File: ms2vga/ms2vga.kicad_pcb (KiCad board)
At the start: 2 copper layers, 34.3 x 31.8 mm, 2 parts, among them J1 DB9_Male_MountingHoles, J2 DB15_Female_HighDensity_Mount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

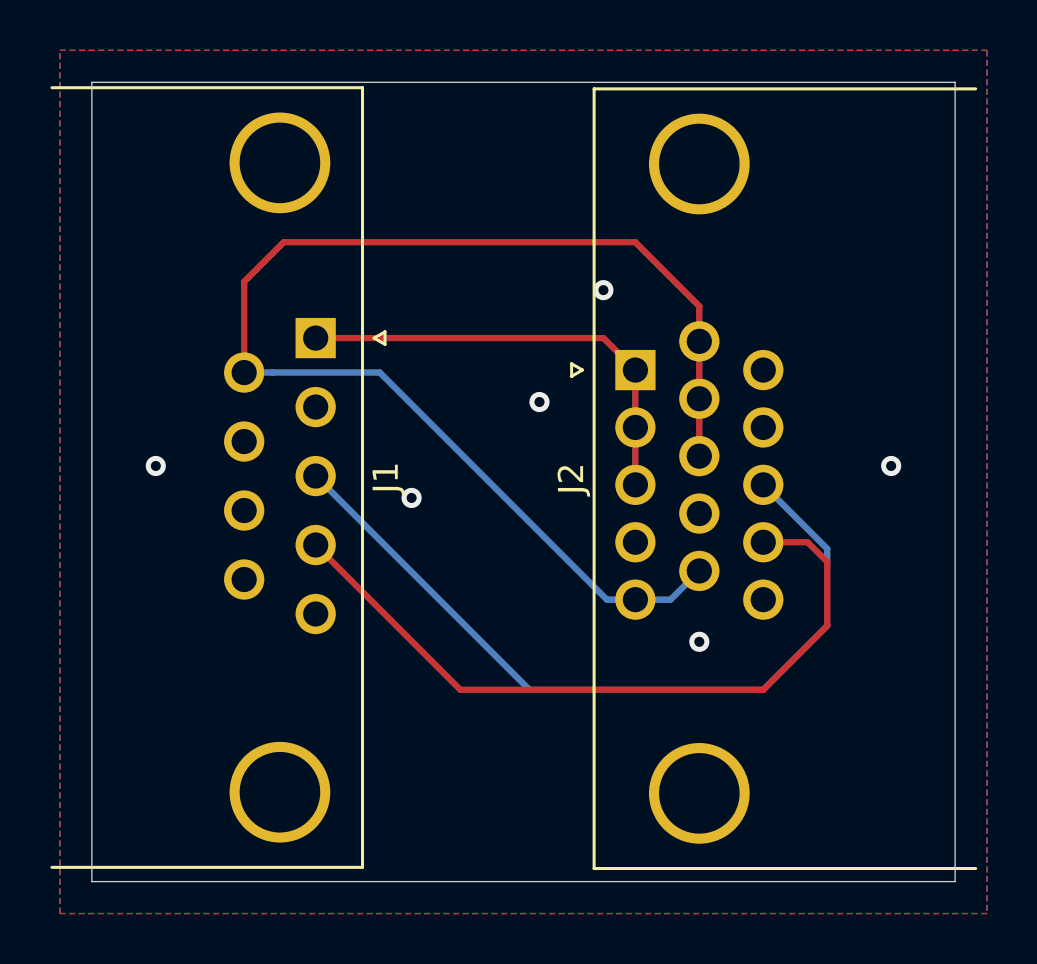
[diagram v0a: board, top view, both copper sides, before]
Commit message: Minor cleanup.
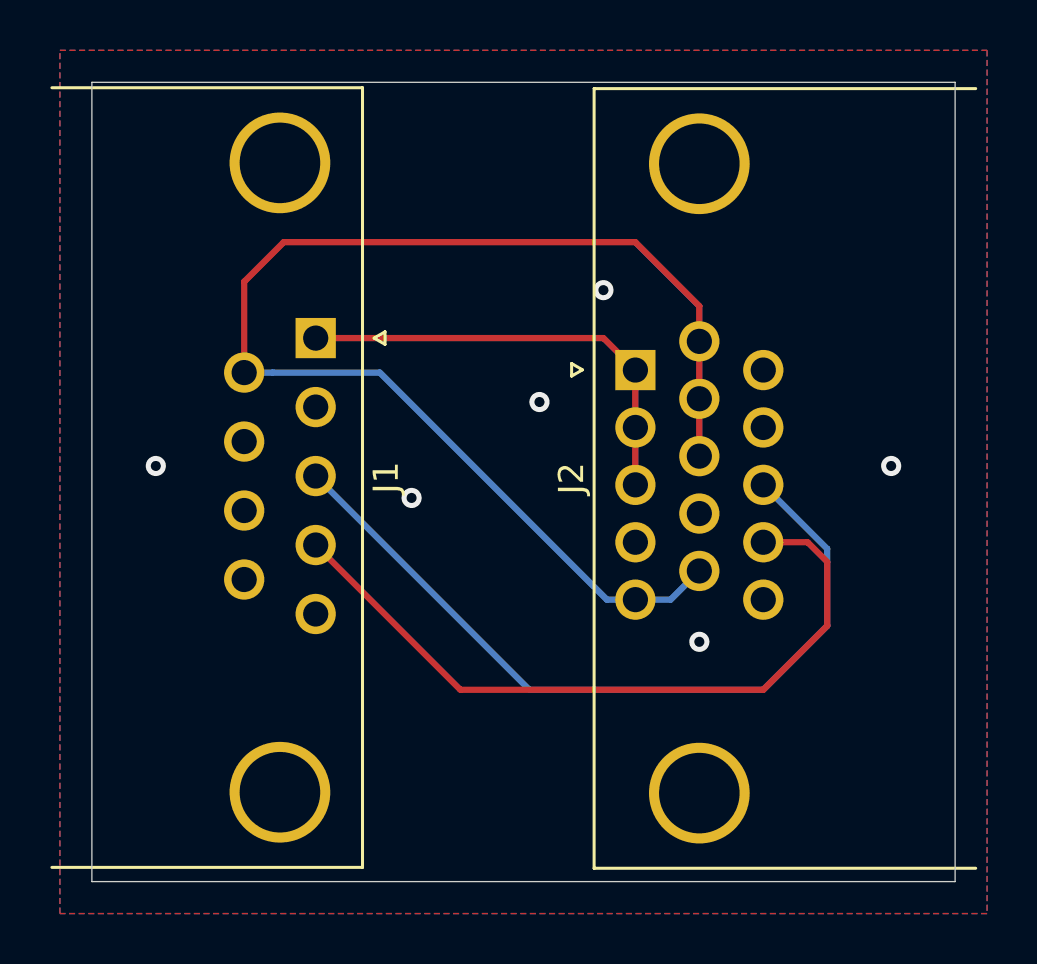
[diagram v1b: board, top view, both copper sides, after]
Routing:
- net Net-(J2-Pad9): vias 0 -> 1
- net /GND: vias 0 -> 1
- net /Chassis: vias 6 -> 4
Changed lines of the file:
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@@
   (general
     (thickness 1.6)
-    (drawings 4)
+    (drawings 6)
     (tracks 34)
     (zones 0)
@@
     (descr "15-pin D-Sub connector, horizontal/angled (90 deg), THT-mount, female, pitch 2.29x1.98mm, pin-PCB-offset 8.35mm, distance of mounting holes 25mm, distance of mounting holes to PCB edge 10.889999999999999mm, see https://disti-assets.s3.amazonaws.com/tonar/files/datasheets/16730.pdf")
     (tags "15-pin D-Sub connector horizontal angled 90deg THT female pitch 2.29x1.98mm pin-PCB-offset 8.35mm mounting-holes-distance 25mm mounting-hole-offset 25mm")
-    (fp_text reference J2 (at -4.315 -2.54 90) (layer F.SilkS)
-      (effects (font (size 1 1) (thickness 0.15)))
-    )
-    (fp_text value DB15_Female_HighDensity_MountingHoles (at -4.315 21.48 90) (layer F.Fab)
-      (effects (font (size 1 1) (thickness 0.15)))
-    )
-    (fp_text user %R (at -4.315 16.98 90) (layer F.Fab)
-      (effects (font (size 1 1) (thickness 0.15)))
-    )
-    (fp_line (start 11.65 -2.1) (end -20.25 -2.1) (layer F.CrtYd) (width 0.05))
-    (fp_line (start 11.65 20.52) (end 11.65 -2.1) (layer F.CrtYd) (width 0.05))
-    (fp_line (start -20.25 20.52) (end 11.65 20.52) (layer F.CrtYd) (width 0.05))
-    (fp_line (start -20.25 -2.1) (end -20.25 20.52) (layer F.CrtYd) (width 0.05))
-    (fp_line (start 0 -2.101325) (end -0.25 -2.534338) (layer F.SilkS) (width 0.12))
-    (fp_line (start 0.25 -2.534338) (end 0 -2.101325) (layer F.SilkS) (width 0.12))
-    (fp_line (start -0.25 -2.534338) (end 0.25 -2.534338) (layer F.SilkS) (width 0.12))
-    (fp_line (start 11.17 -1.64) (end 11.17 13.52) (layer F.SilkS) (width 0.12))
-    (fp_line (start -19.8 -1.64) (end 11.17 -1.64) (layer F.SilkS) (width 0.12))
-    (fp_line (start -19.8 13.52) (end -19.8 -1.64) (layer F.SilkS) (width 0.12))
-    (fp_line (start 9.785 13.58) (end 9.785 2.69) (layer F.Fab) (width 0.1))
-    (fp_line (start 6.585 13.58) (end 6.585 2.69) (layer F.Fab) (width 0.1))
-    (fp_line (start -15.215 13.58) (end -15.215 2.69) (layer F.Fab) (width 0.1))
-    (fp_line (start -18.415 13.58) (end -18.415 2.69) (layer F.Fab) (width 0.1))
-    (fp_line (start 10.685 13.98) (end 5.685 13.98) (layer F.Fab) (width 0.1))
-    (fp_line (start 10.685 18.98) (end 10.685 13.98) (layer F.Fab) (width 0.1))
-    (fp_line (start 5.685 18.98) (end 10.685 18.98) (layer F.Fab) (width 0.1))
-    (fp_line (start 5.685 13.98) (end 5.685 18.98) (layer F.Fab) (width 0.1))
-    (fp_line (start -14.315 13.98) (end -19.315 13.98) (layer F.Fab) (width 0.1))
-    (fp_line (start -14.315 18.98) (end -14.315 13.98) (layer F.Fab) (width 0.1))
-    (fp_line (start -19.315 18.98) (end -14.315 18.98) (layer F.Fab) (width 0.1))
-    (fp_line (start -19.315 13.98) (end -19.315 18.98) (layer F.Fab) (width 0.1))
-    (fp_line (start 3.835 13.98) (end -12.465 13.98) (layer F.Fab) (width 0.1))
-    (fp_line (start 3.835 19.98) (end 3.835 13.98) (layer F.Fab) (width 0.1))
-    (fp_line (start -12.465 19.98) (end 3.835 19.98) (layer F.Fab) (width 0.1))
-    (fp_line (start -12.465 13.98) (end -12.465 19.98) (layer F.Fab) (width 0.1))
-    (fp_line (start 11.11 13.58) (end -19.74 13.58) (layer F.Fab) (width 0.1))
-    (fp_line (start 11.11 13.98) (end 11.11 13.58) (layer F.Fab) (width 0.1))
-    (fp_line (start -19.74 13.98) (end 11.11 13.98) (layer F.Fab) (width 0.1))
-    (fp_line (start -19.74 13.58) (end -19.74 13.98) (layer F.Fab) (width 0.1))
-    (fp_line (start 11.11 -1.58) (end -19.74 -1.58) (layer F.Fab) (width 0.1))
-    (fp_line (start 11.11 13.58) (end 11.11 -1.58) (layer F.Fab) (width 0.1))
-    (fp_line (start -19.74 13.58) (end 11.11 13.58) (layer F.Fab) (width 0.1))
-    (fp_line (start -19.74 -1.58) (end -19.74 13.58) (layer F.Fab) (width 0.1))
-    (fp_arc (start 8.185 2.69) (end 6.585 2.69) (angle 180) (layer F.Fab) (width 0.1))
-    (fp_arc (start -16.815 2.69) (end -18.415 2.69) (angle 180) (layer F.Fab) (width 0.1))
-    (pad 0 thru_hole circle (at 8.185 2.54 90) (size 4 4) (drill 3.2) (layers *.Cu *.Mask)
+    (fp_text reference J2 (at -4.305 -2.54 90) (layer F.SilkS)
+      (effects (font (size 1 1) (thickness 0.15)))
+    )
+    (fp_text value DB15_Female_HighDensity_MountingHoles (at -4.305 21.48 90) (layer F.Fab)
+      (effects (font (size 1 1) (thickness 0.15)))
+    )
+    (fp_text user %R (at -4.305 16.98 90) (layer F.Fab)
+      (effects (font (size 1 1) (thickness 0.15)))
+    )
+    (fp_line (start 11.66 -2.1) (end -20.24 -2.1) (layer F.CrtYd) (width 0.05))
+    (fp_line (start 11.66 20.52) (end 11.66 -2.1) (layer F.CrtYd) (width 0.05))
+    (fp_line (start -20.24 20.52) (end 11.66 20.52) (layer F.CrtYd) (width 0.05))
+    (fp_line (start -20.24 -2.1) (end -20.24 20.52) (layer F.CrtYd) (width 0.05))
+    (fp_line (start 0.01 -2.101325) (end -0.24 -2.534338) (layer F.SilkS) (width 0.12))
+    (fp_line (start 0.26 -2.534338) (end 0.01 -2.101325) (layer F.SilkS) (width 0.12))
+    (fp_line (start -0.24 -2.534338) (end 0.26 -2.534338) (layer F.SilkS) (width 0.12))
+    (fp_line (start 11.18 -1.64) (end 11.18 13.52) (layer F.SilkS) (width 0.12))
+    (fp_line (start -19.79 -1.64) (end 11.18 -1.64) (layer F.SilkS) (width 0.12))
+    (fp_line (start -19.79 13.52) (end -19.79 -1.64) (layer F.SilkS) (width 0.12))
+    (fp_line (start 9.795 13.58) (end 9.795 2.69) (layer F.Fab) (width 0.1))
+    (fp_line (start 6.595 13.58) (end 6.595 2.69) (layer F.Fab) (width 0.1))
+    (fp_line (start -15.205 13.58) (end -15.205 2.69) (layer F.Fab) (width 0.1))
+    (fp_line (start -18.405 13.58) (end -18.405 2.69) (layer F.Fab) (width 0.1))
+    (fp_line (start 10.695 13.98) (end 5.695 13.98) (layer F.Fab) (width 0.1))
+    (fp_line (start 10.695 18.98) (end 10.695 13.98) (layer F.Fab) (width 0.1))
+    (fp_line (start 5.695 18.98) (end 10.695 18.98) (layer F.Fab) (width 0.1))
+    (fp_line (start 5.695 13.98) (end 5.695 18.98) (layer F.Fab) (width 0.1))
+    (fp_line (start -14.305 13.98) (end -19.305 13.98) (layer F.Fab) (width 0.1))
+    (fp_line (start -14.305 18.98) (end -14.305 13.98) (layer F.Fab) (width 0.1))
+    (fp_line (start -19.305 18.98) (end -14.305 18.98) (layer F.Fab) (width 0.1))
+    (fp_line (start -19.305 13.98) (end -19.305 18.98) (layer F.Fab) (width 0.1))
+    (fp_line (start 3.845 13.98) (end -12.455 13.98) (layer F.Fab) (width 0.1))
+    (fp_line (start 3.845 19.98) (end 3.845 13.98) (layer F.Fab) (width 0.1))
+    (fp_line (start -12.455 19.98) (end 3.845 19.98) (layer F.Fab) (width 0.1))
+    (fp_line (start -12.455 13.98) (end -12.455 19.98) (layer F.Fab) (width 0.1))
+    (fp_line (start 11.12 13.58) (end -19.73 13.58) (layer F.Fab) (width 0.1))
+    (fp_line (start 11.12 13.98) (end 11.12 13.58) (layer F.Fab) (width 0.1))
+    (fp_line (start -19.73 13.98) (end 11.12 13.98) (layer F.Fab) (width 0.1))
+    (fp_line (start -19.73 13.58) (end -19.73 13.98) (layer F.Fab) (width 0.1))
+    (fp_line (start 11.12 -1.58) (end -19.73 -1.58) (layer F.Fab) (width 0.1))
+    (fp_line (start 11.12 13.58) (end 11.12 -1.58) (layer F.Fab) (width 0.1))
+    (fp_line (start -19.73 13.58) (end 11.12 13.58) (layer F.Fab) (width 0.1))
+    (fp_line (start -19.73 -1.58) (end -19.73 13.58) (layer F.Fab) (width 0.1))
+    (fp_arc (start 8.195 2.69) (end 6.595 2.69) (angle 180) (layer F.Fab) (width 0.1))
+    (fp_arc (start -16.805 2.69) (end -18.405 2.69) (angle 180) (layer F.Fab) (width 0.1))
+    (pad 0 thru_hole circle (at 8.195 2.54 90) (size 4 4) (drill 3.2) (layers *.Cu *.Mask)
       (net 10 /Chassis))
-    (pad 0 thru_hole circle (at -16.815 2.54 90) (size 4 4) (drill 3.2) (layers *.Cu *.Mask)
+    (pad 0 thru_hole circle (at -16.805 2.54 90) (size 4 4) (drill 3.2) (layers *.Cu *.Mask)
       (net 10 /Chassis))
     (pad 15 thru_hole circle (at -9.12 5.08 90) (size 1.6 1.6) (drill 1) (layers *.Cu *.Mask)
@@
     )
   )
+  (gr_poly (pts (xy 125.73 81.28) (xy 128.27 81.28) (xy 128.27 113.03) (xy 125.73 113.03)) (layer Cmts.User) (width 0.1))
+  (gr_poly (pts (xy 162.56 81.28) (xy 163.83 81.28) (xy 163.83 113.03) (xy 162.56 113.03)) (layer Cmts.User) (width 0.1))
   (gr_line (start 128.27 113.03) (end 128.27 81.28) (layer Edge.Cuts) (width 0.05))
   (gr_line (start 162.56 113.03) (end 128.27 113.03) (layer Edge.Cuts) (width 0.05))
@@
   (segment (start 148.72863 101.83) (end 139.70863 92.81) (width 0.25) (layer B.Cu) (net 6))
   (segment (start 149.86 101.83) (end 148.72863 101.83) (width 0.25) (layer B.Cu) (net 6))
+  (via (at 140.97 97.79) (size 0.8) (drill 0.4) (layers F.Cu B.Cu) (net 6))
   (via (at 160.02 96.52) (size 0.8) (drill 0.4) (layers F.Cu B.Cu) (net 10))
   (via (at 130.81 96.52) (size 0.8) (drill 0.4) (layers F.Cu B.Cu) (net 10))
   (via (at 148.59 89.535) (size 0.8) (drill 0.4) (layers F.Cu B.Cu) (net 10))
-  (via (at 152.4 103.505) (size 0.8) (drill 0.4) (layers F.Cu B.Cu) (net 10))
-  (via (at 140.97 97.79) (size 0.8) (drill 0.4) (layers F.Cu B.Cu) (net 10))
   (via (at 146.05 93.98) (size 0.8) (drill 0.4) (layers F.Cu B.Cu) (net 10))
+  (via (at 152.4 103.505) (size 0.8) (drill 0.4) (layers F.Cu B.Cu) (net 14))
   (zone (net 10) (net_name /Chassis) (layer F.Cu) (hatch edge 0.508)
     (connect_pads (clearance 0.508))
